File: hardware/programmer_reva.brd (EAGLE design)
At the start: 30 x 21 mm, 2 parts

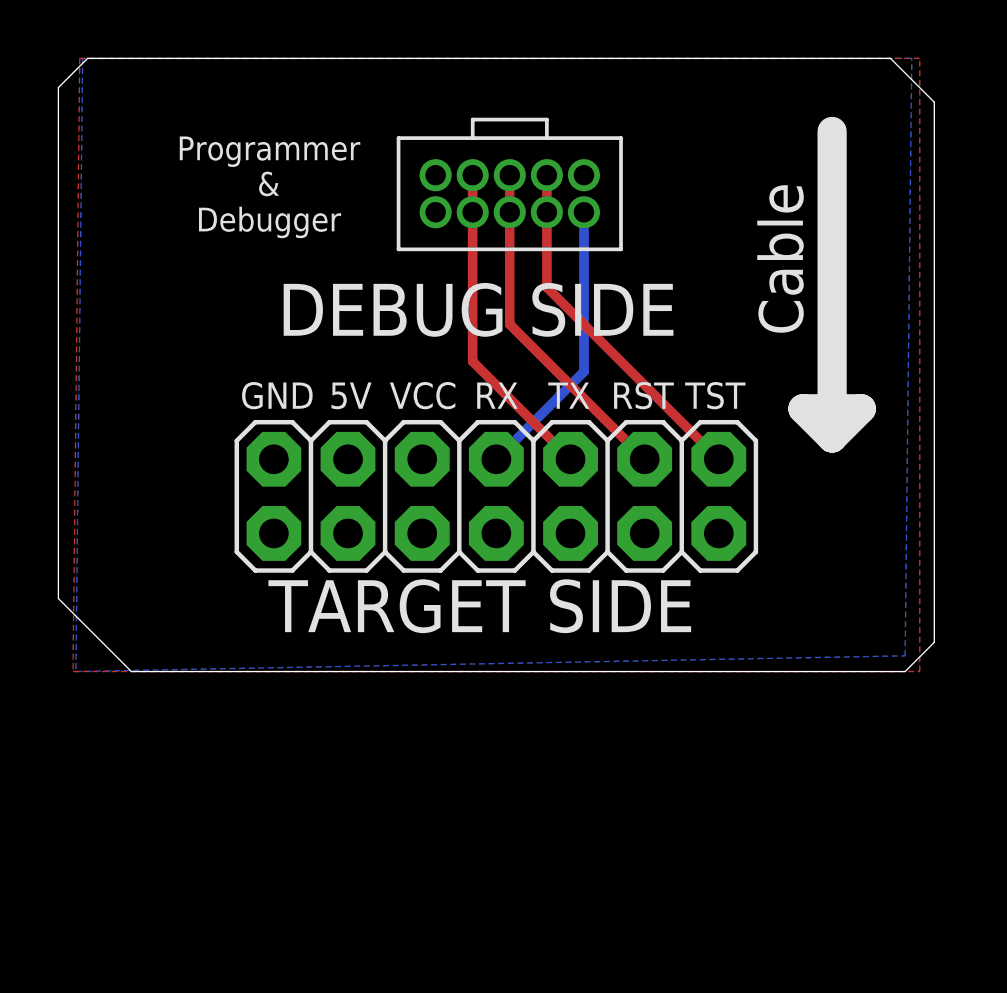
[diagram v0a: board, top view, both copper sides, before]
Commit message: final hardware files, already sent to fab
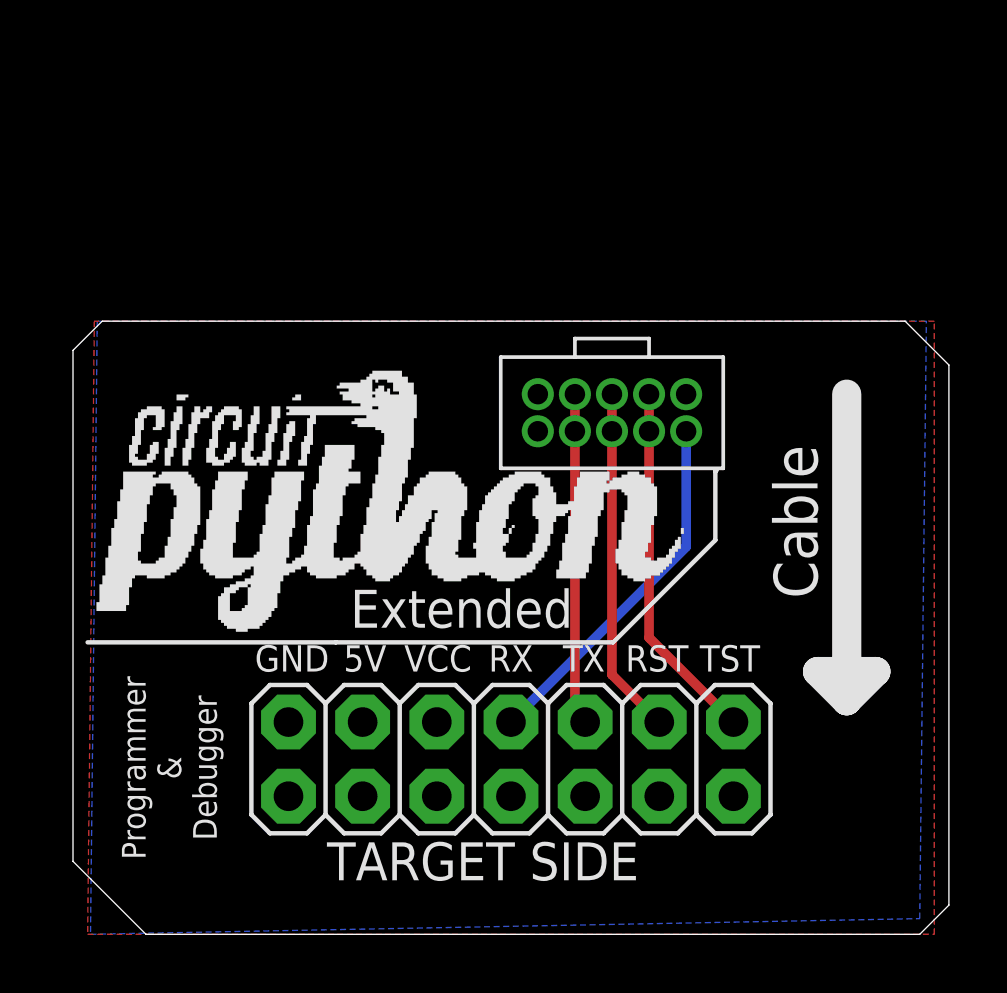
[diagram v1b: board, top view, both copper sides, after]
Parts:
- added U$1: (no value), northwestern-logo:NU-LOGO
- added U$2: LOGO, circuitpython-logo:CIRCUITPYTHON-LOGO
- moved JP1 9.01 mm to (15.0, 6.00)
- moved JP2 8.28 mm to (21.0, 18.5)
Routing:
- net RX_DEBUG: track 9.70 -> 12.4 mm
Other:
- board text added: "Extended"
- board text removed: "DEBUG SIDE"
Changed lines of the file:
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@@
 <board>
 <plain>
-<text x="11" y="21.5" size="0.7" layer="22" font="fixed" rot="MR180">Programmer Rev. A
+<text x="11.5" y="12.5" size="0.7" layer="22" font="fixed" rot="MR180">Programmer Rev. A
 Josiah Hester
 Northwestern University
 </text>
-<text x="6.7" y="25.7" size="0.8128" layer="21" font="fixed" align="center">Programmer
+<text x="3.3" y="5.7" size="0.8128" layer="21" font="vector" ratio="13" rot="R90" align="center">Programmer
 &amp;
 Debugger</text>
-<wire x1="-0.5" y1="29" x2="0.5" y2="30" width="0.001" layer="20"/>
-<wire x1="0.5" y1="30" x2="28" y2="30" width="0.001" layer="20"/>
-<wire x1="28" y1="30" x2="29.5" y2="28.5" width="0.001" layer="20"/>
-<wire x1="29.5" y1="28.5" x2="29.5" y2="10" width="0.001" layer="20"/>
-<wire x1="29.5" y1="10" x2="28.5" y2="9" width="0.001" layer="20"/>
-<wire x1="28.5" y1="9" x2="2" y2="9" width="0.001" layer="20"/>
-<wire x1="2" y1="9" x2="-0.5" y2="11.5" width="0.001" layer="20"/>
-<wire x1="-0.5" y1="11.5" x2="-0.5" y2="29" width="0.001" layer="20"/>
-<text x="7" y="20.5" size="1.778" layer="21" font="fixed">DEBUG SIDE</text>
-<text x="6.7" y="10.35" size="1.778" layer="21" font="fixed">TARGET SIDE</text>
-<text x="7" y="18" size="0.9" layer="21" font="fixed" align="bottom-center">GND</text>
-<text x="9.5" y="18" size="0.9" layer="21" font="fixed" align="bottom-center">5V</text>
-<text x="12" y="18" size="0.9" layer="21" font="fixed" align="bottom-center">VCC</text>
-<text x="14.5" y="18" size="0.9" layer="21" font="fixed" align="bottom-center">RX</text>
-<text x="17" y="18" size="0.9" layer="21" font="fixed" align="bottom-center">TX</text>
-<text x="19.5" y="18" size="0.9" layer="21" font="fixed" align="bottom-center">RST</text>
-<text x="22" y="18" size="0.9" layer="21" font="fixed" align="bottom-center">TST</text>
-<wire x1="26" y1="27.5" x2="26" y2="17" width="1" layer="21"/>
-<wire x1="26" y1="17" x2="27" y2="18" width="1" layer="21"/>
-<wire x1="27" y1="18" x2="25" y2="18" width="1" layer="21"/>
-<wire x1="25" y1="18" x2="26" y2="17" width="1" layer="21"/>
-<text x="25" y="20.5" size="1.5" layer="21" font="vector" ratio="17" rot="R90">Cable</text>
+<wire x1="0" y1="20" x2="1" y2="21" width="0.001" layer="20"/>
+<wire x1="1" y1="21" x2="28.5" y2="21" width="0.001" layer="20"/>
+<wire x1="28.5" y1="21" x2="30" y2="19.5" width="0.001" layer="20"/>
+<wire x1="30" y1="19.5" x2="30" y2="1" width="0.001" layer="20"/>
+<wire x1="30" y1="1" x2="29" y2="0" width="0.001" layer="20"/>
+<wire x1="29" y1="0" x2="2.5" y2="0" width="0.001" layer="20"/>
+<wire x1="2.5" y1="0" x2="0" y2="2.5" width="0.001" layer="20"/>
+<wire x1="0" y1="2.5" x2="0" y2="20" width="0.001" layer="20"/>
+<text x="8.7" y="1.85" size="1.3" layer="21" font="vector" ratio="13">TARGET SIDE</text>
+<text x="7.5" y="9" size="0.9" layer="21" font="fixed" align="bottom-center">GND</text>
+<text x="10" y="9" size="0.9" layer="21" font="fixed" align="bottom-center">5V</text>
+<text x="12.5" y="9" size="0.9" layer="21" font="fixed" align="bottom-center">VCC</text>
+<text x="15" y="9" size="0.9" layer="21" font="fixed" align="bottom-center">RX</text>
+<text x="17.5" y="9" size="0.9" layer="21" font="fixed" align="bottom-center">TX</text>
+<text x="20" y="9" size="0.9" layer="21" font="fixed" align="bottom-center">RST</text>
+<text x="22.5" y="9" size="0.9" layer="21" font="fixed" align="bottom-center">TST</text>
+<wire x1="26.5" y1="18.5" x2="26.5" y2="8" width="1" layer="21"/>
+<wire x1="26.5" y1="8" x2="27.5" y2="9" width="1" layer="21"/>
+<wire x1="27.5" y1="9" x2="25.5" y2="9" width="1" layer="21"/>
+<wire x1="25.5" y1="9" x2="26.5" y2="8" width="1" layer="21"/>
+<text x="25.5" y="11.5" size="1.5" layer="21" font="vector" ratio="17" rot="R90">Cable</text>
+<text x="9.5" y="10.5" size="1.3" layer="21" font="vector" ratio="18">Extended</text>
+<wire x1="9" y1="10" x2="18.5" y2="10" width="0.1524" layer="21"/>
+<wire x1="18.5" y1="10" x2="22" y2="13.5" width="0.1524" layer="21"/>
+<wire x1="22" y1="13.5" x2="22" y2="15.85" width="0.1524" layer="21"/>
+<wire x1="22" y1="15.85" x2="22.05" y2="15.9" width="0.1524" layer="21"/>
+<wire x1="9" y1="10" x2="0.5" y2="10" width="0.1524" layer="21"/>
 </plain>
 <attributes>
@@
 </autorouter>
 <elements>
-<element name="JP1" library="SparkFun-Connectors" package="2X7" value="M07X2" x="14.5" y="15" rot="R180"/>
-<element name="JP2" library="SparkFun-Connectors" package="2X5_1.27MM" value="" x="17.5" y="26" rot="R270">
-<attribute name="DIGIKEY" value="1175-1627-ND " x="25.5" y="31" size="1.5" layer="27" font="vector" ratio="17" rot="R270" display="off"/>
+<element name="JP1" library="SparkFun-Connectors" package="2X7" value="M07X2" x="15" y="6" rot="R180"/>
+<element name="JP2" library="SparkFun-Connectors" package="2X5_1.27MM" value="" x="21" y="18.5" rot="R270">
+<attribute name="DIGIKEY" value="1175-1627-ND " x="29" y="23.5" size="1.5" layer="27" font="vector" ratio="17" rot="R270" display="off"/>
 </element>
+<element name="U$1" library="northwestern-logo" package="NU-LOGO" value="" x="11" y="10" rot="MR0"/>
+<element name="U$2" library="circuitpython-logo" package="CIRCUITPYTHON-LOGO" value="LOGO" x="0.65" y="9.6"/>
 </elements>
 <signals>
 <signal name="GND">
 <polygon width="0.3048" layer="1">
-<vertex x="0" y="9"/>
-<vertex x="29" y="9"/>
-<vertex x="29" y="30"/>
-<vertex x="0.23076875" y="30"/>
+<vertex x="0.5" y="0"/>
+<vertex x="29.5" y="0"/>
+<vertex x="29.5" y="21"/>
+<vertex x="0.73076875" y="21"/>
 </polygon>
 <contactref element="JP1" pad="13"/>
@@
 <signal name="VCC">
 <polygon width="0.3048" layer="16">
-<vertex x="0.098921875" y="9.001865625"/>
-<vertex x="28.50041875" y="9.53774375"/>
-<vertex x="28.727778125" y="30"/>
-<vertex x="0.32966875" y="30"/>
+<vertex x="0.598921875" y="0.001865625"/>
+<vertex x="29.00041875" y="0.53774375"/>
+<vertex x="29.227778125" y="21"/>
+<vertex x="0.82966875" y="21"/>
 </polygon>
 <contactref element="JP1" pad="9"/>
@@
 <contactref element="JP2" pad="3"/>
 <contactref element="JP2" pad="4"/>
-<wire x1="22.12" y1="16.27" x2="16.23" y2="22.16" width="0.3302" layer="1"/>
-<wire x1="16.23" y1="22.16" x2="16.23" y2="24.73" width="0.3302" layer="1"/>
-<wire x1="16.23" y1="26" x2="16.23" y2="24.73" width="0.3302" layer="1"/>
+<wire x1="22.62" y1="7.27" x2="19.73" y2="10.16" width="0.3302" layer="1"/>
+<wire x1="19.73" y1="10.16" x2="19.73" y2="17.23" width="0.3302" layer="1"/>
+<wire x1="19.73" y1="18.5" x2="19.73" y2="17.23" width="0.3302" layer="1"/>
 </signal>
 <signal name="MSP430_RST">
@@
 <contactref element="JP2" pad="5"/>
 <contactref element="JP2" pad="6"/>
-<wire x1="19.58" y1="16.27" x2="14.96" y2="20.89" width="0.3302" layer="1"/>
-<wire x1="14.96" y1="20.89" x2="14.96" y2="24.73" width="0.3302" layer="1"/>
-<wire x1="14.96" y1="24.73" x2="14.96" y2="26" width="0.3302" layer="1"/>
+<wire x1="20.08" y1="7.27" x2="18.46" y2="8.89" width="0.3302" layer="1"/>
+<wire x1="18.46" y1="8.89" x2="18.46" y2="17.23" width="0.3302" layer="1"/>
+<wire x1="18.46" y1="17.23" x2="18.46" y2="18.5" width="0.3302" layer="1"/>
 </signal>
 <signal name="VL">
@@
 <contactref element="JP2" pad="7"/>
 <contactref element="JP2" pad="8"/>
-<wire x1="17.04" y1="16.27" x2="13.69" y2="19.62" width="0.3302" layer="1"/>
-<wire x1="13.69" y1="19.62" x2="13.69" y2="24.73" width="0.3302" layer="1"/>
-<wire x1="13.69" y1="24.73" x2="13.69" y2="26" width="0.3302" layer="1"/>
+<wire x1="17.54" y1="7.27" x2="17.19" y2="7.62" width="0.3302" layer="1"/>
+<wire x1="17.19" y1="7.62" x2="17.19" y2="17.23" width="0.3302" layer="1"/>
+<wire x1="17.19" y1="17.23" x2="17.19" y2="18.5" width="0.3302" layer="1"/>
 </signal>
 <signal name="RX_DEBUG">
 <contactref element="JP1" pad="7"/>
 <contactref element="JP2" pad="2"/>
-<wire x1="14.5" y1="16.27" x2="17.5" y2="19.27" width="0.3302" layer="16"/>
-<wire x1="17.5" y1="19.27" x2="17.5" y2="24.73" width="0.3302" layer="16"/>
+<wire x1="15" y1="7.27" x2="21" y2="13.27" width="0.3302" layer="16"/>
+<wire x1="21" y1="13.27" x2="21" y2="17.23" width="0.3302" layer="16"/>
 </signal>
 <signal name="5V">
